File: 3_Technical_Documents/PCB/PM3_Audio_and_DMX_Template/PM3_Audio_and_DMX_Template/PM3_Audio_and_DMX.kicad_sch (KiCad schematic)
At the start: 9 parts, among them J1 DMX-out

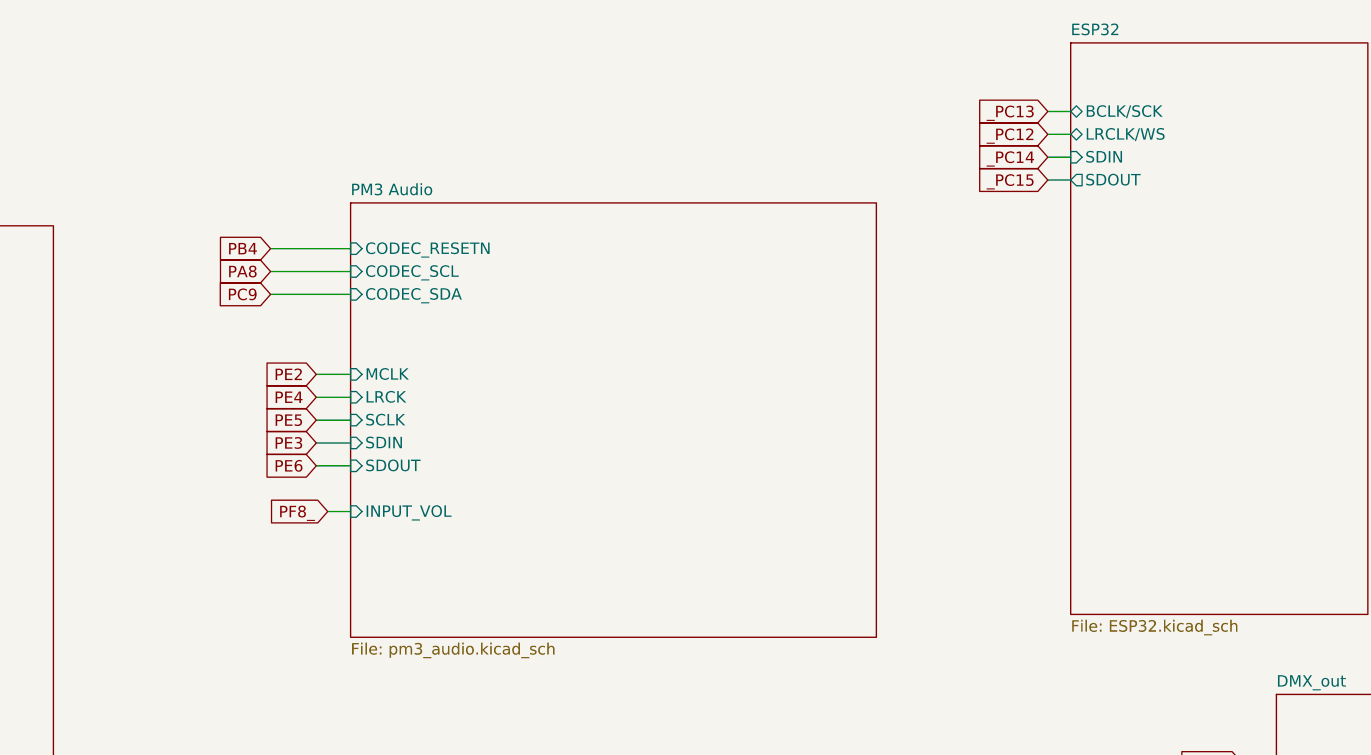
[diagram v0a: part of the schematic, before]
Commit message: esp-stm connection (+ conflict recolution)
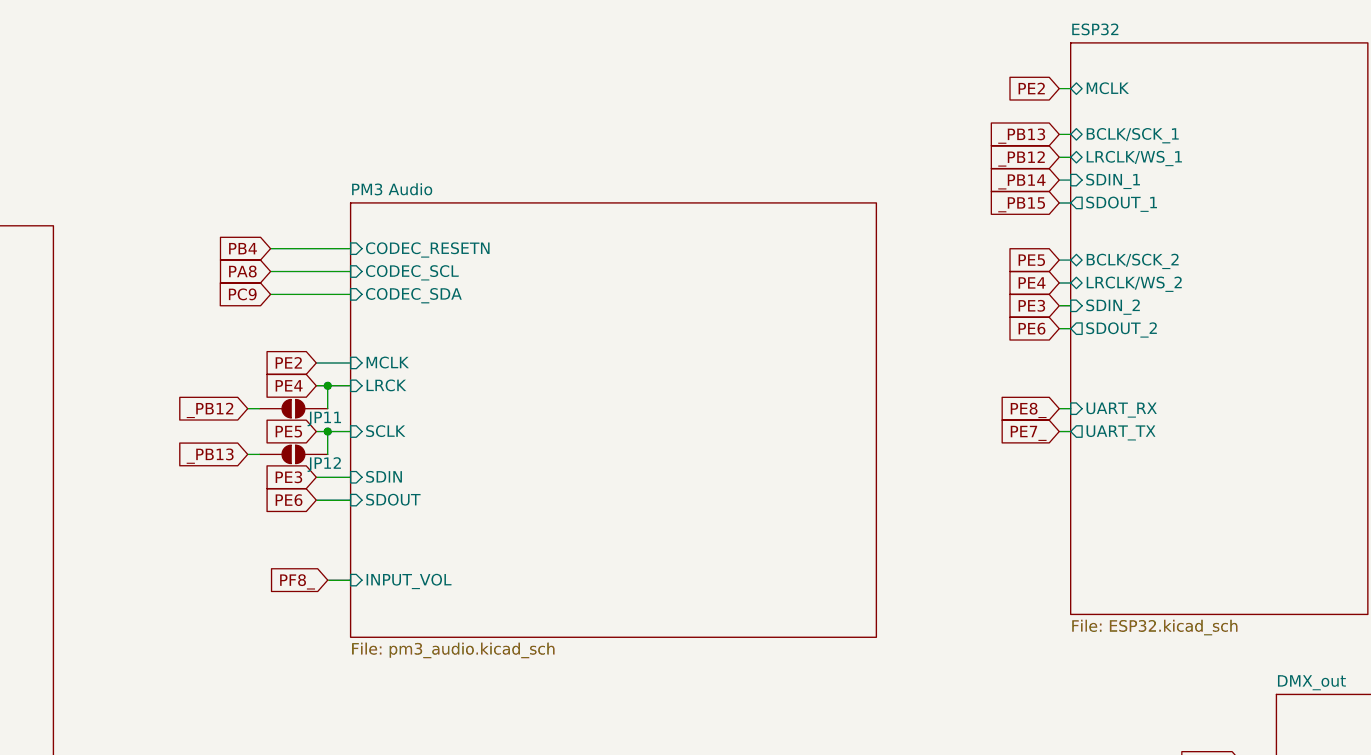
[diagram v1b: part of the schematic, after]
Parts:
- added JP11, JP12: SolderJumper_2_Open, Jumper:SolderJumper-2_P1.3mm_Open_RoundedPad1.0x1.5mm, symbol Jumper:SolderJumper_2_Open
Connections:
- net PE4: now also JP11.2 (B)
- net PE5: now also JP12.2 (B)
- new net _PB12: JP11.1 (A)
- new net _PB13: JP12.1 (A)
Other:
- sheet ESP32 ports: added BCLK/SCK_1, BCLK/SCK_2, LRCLK/WS_1, LRCLK/WS_2, MCLK, SDIN_1, SDIN_2, SDOUT_1, SDOUT_2, UART_RX, UART_TX; removed BCLK/SCK, LRCLK/WS, SDIN, SDOUT
